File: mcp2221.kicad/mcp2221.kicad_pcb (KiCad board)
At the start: 2 copper layers, 71.5 x 45.4 mm, 24 parts, among them J1 Conn_01x07_Male, J2 Jumper 32 or 21, J3 Conn_01x02_Male, J4 Conn_01x02_Male, J5 Conn_01x04_Male, J6 Conn_01x03_Male, J7 Conn_01x03_Male, SW1 SW_Push, U1 AMS1117CD-3.3, U2 MCP2221

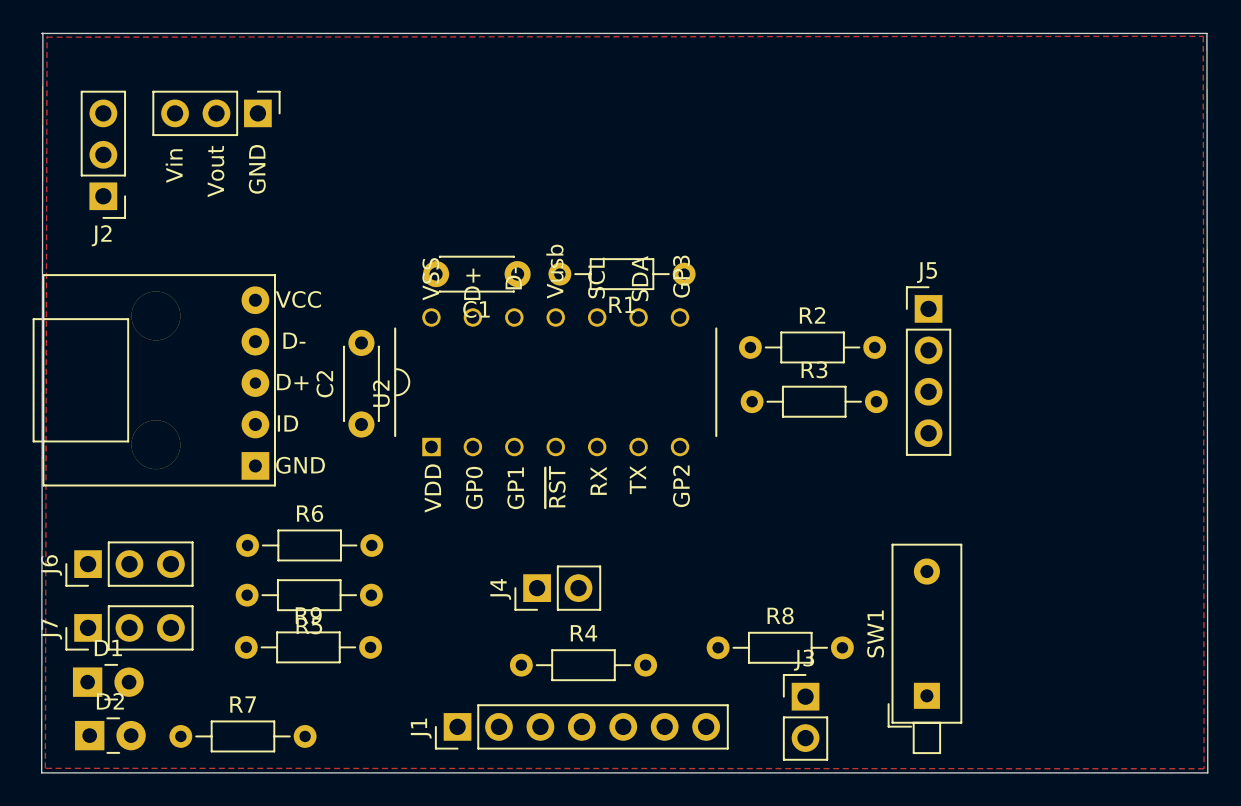
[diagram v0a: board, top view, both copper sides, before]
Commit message: pcb layout changes
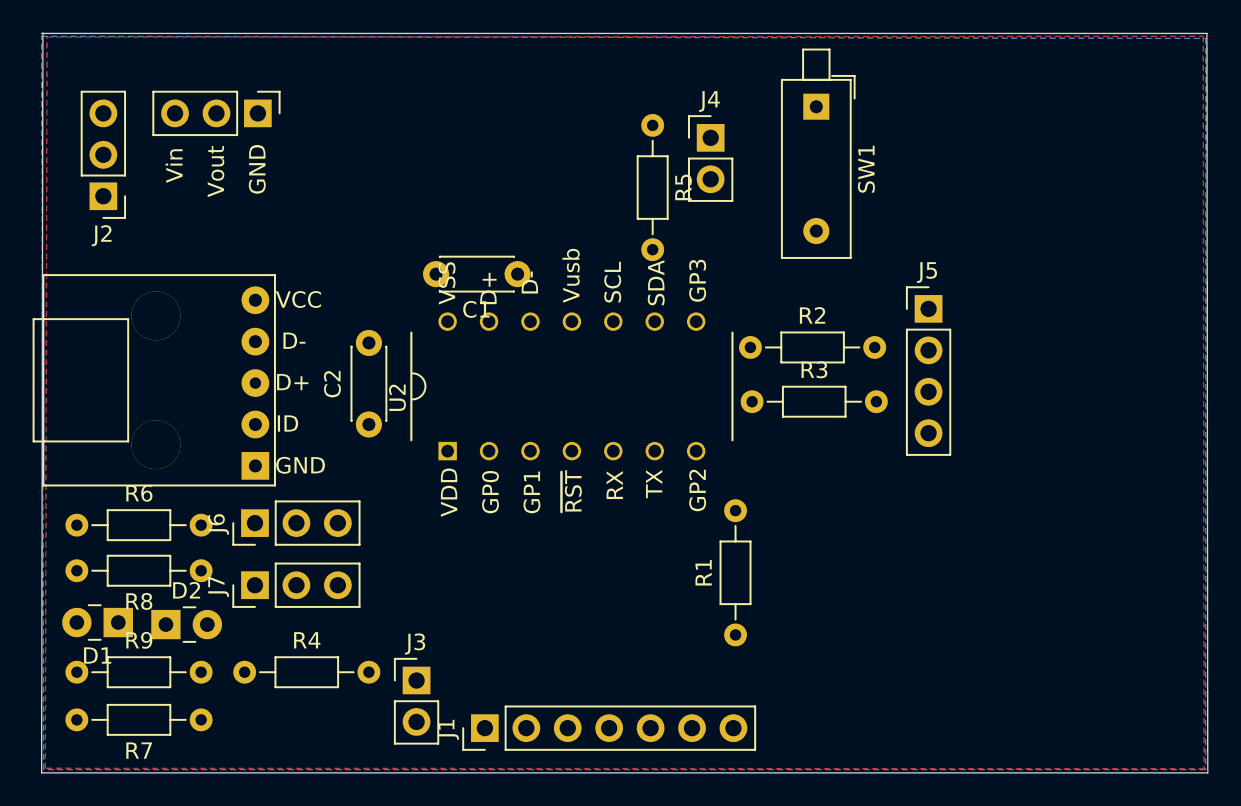
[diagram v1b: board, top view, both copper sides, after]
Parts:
- moved SW1 36.7 mm to (111.8, 48.0), turned to 270 degrees
- moved R5 33.6 mm to (101.7, 49.1), turned to 270 degrees
- moved R8 32.0 mm to (74.0, 76.5), turned to 180 degrees
- moved J4 29.6 mm to (105.3, 49.9), turned to 0 degrees
- moved J3 23.9 mm to (87.2, 83.2)
- moved R1 22.3 mm to (106.8, 80.4), turned to 90 degrees
- moved R4 17.0 mm to (76.7, 82.7)
- moved J7 10.6 mm to (77.3, 77.3)
- moved J6 10.5 mm to (77.3, 73.5)
- moved R6 10.5 mm to (66.4, 73.7)
- moved R9 10.5 mm to (66.4, 82.7)
- moved D2 8.26 mm to (71.9, 79.8)
- moved D1 4.11 mm to (69.0, 79.6), turned to 180 degrees
- moved J1 1.68 mm to (91.4, 86.1)
- moved R7 1.61 mm to (74.0, 85.6), turned to 180 degrees
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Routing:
- added copper zone on B.Cu, net GND
